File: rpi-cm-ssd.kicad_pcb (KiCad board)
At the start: 4 copper layers, 107 x 55.9 mm, 153 parts, among them J1 ARJM11B1-502-AB-EW2, J2 Bus_M.2_Socket_M, J3 USB_C_Receptacle, J4 PD controller EEPROM programm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, J5 690-008-221-904, J6 CONUFL001-SMD-T, Q1 DMG1012T, SW1 SW_DIP_x05, U1 SN74LVC1G11, U10 TPS65283-1RGER, U11 USB2512, U12 24LC32, U13 TCN75AVUA, U14 TCN75AVUA, U15 SN74LVC1G07, U16 MGM210PB32JIA2, U2 TPD4EUSB30, U3 TPD4EUSB30, U4 74LVC1G07, U5 SN74LVC1G3157, U6 CAT24C256, U7 TVS2200DRV, U8 TPS25750DRJKT, U9 PAC1951-1, Y1 24MHz

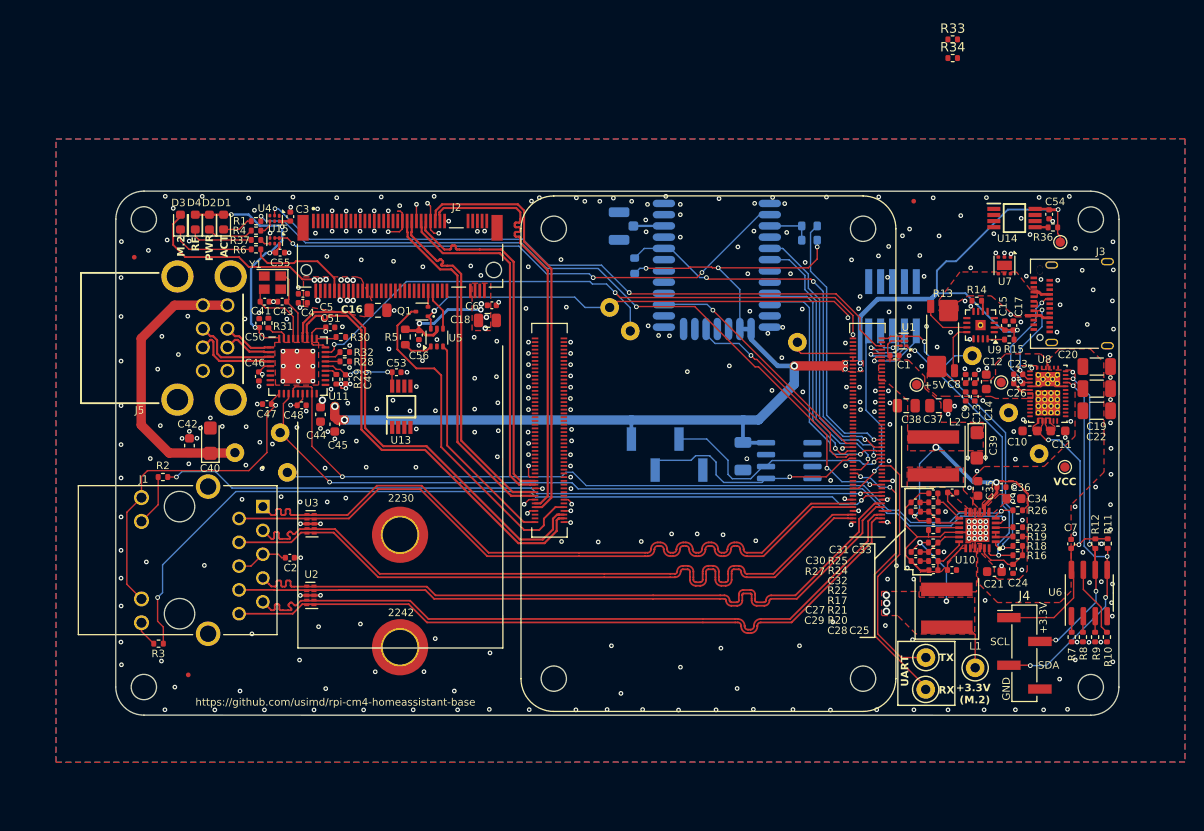
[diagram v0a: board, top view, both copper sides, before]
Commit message: Rev 2
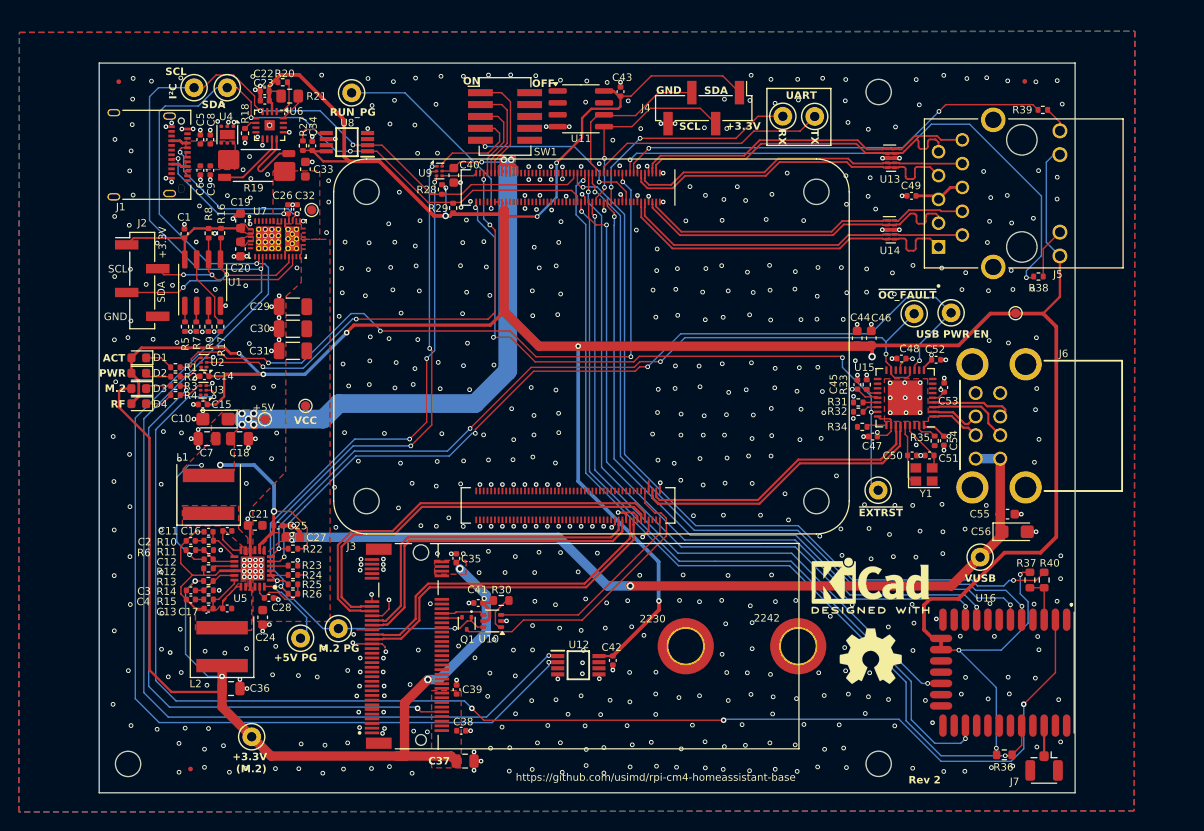
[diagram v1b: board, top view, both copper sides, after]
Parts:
- removed the C12 at (149.8, 50.5)
- removed the C13 at (149.8, 52.4)
- removed the H4 at (61.1, 33.5)
- added C5: 10nF, Capacitor_SMD:C_0402_1005Metric, F.Cu at (67.1, 25.0)
- added C6: 10nF, Capacitor_SMD:C_0402_1005Metric, F.Cu at (67.1, 28.3)
- added R20: 100k, Resistor_SMD:R_0402_1005Metric, F.Cu at (75.9, 18.9)
- added REF**: KiCad-Logo2_5mm_SilkScreen, Symbol:KiCad-Logo2_5mm_SilkScreen, F.Cu at (138.6, 72.6)
- added REF**: OSHW-Symbol_6.7x6mm_SilkScreen, Symbol:OSHW-Symbol_6.7x6mm_SilkScreen, F.Cu at (138.7, 80.1)
- added REF**: WEEE-Logo_4.2x6mm_SilkScreen, Symbol:WEEE-Logo_4.2x6mm_SilkScreen, B.Cu at (132.8, 90.2)
- added REF**: RoHS-Logo_6mm_SilkScreen, Symbol:RoHS-Logo_6mm_SilkScreen, B.Cu at (110.7, 90.4)
- added REF**: ESD-Logo_6.6x6mm_SilkScreen, Symbol:ESD-Logo_6.6x6mm_SilkScreen, B.Cu at (126.0, 90.4)
- added REF**: Symbol_GNU-Logo_SilkscreenTop, Symbol:Symbol_GNU-Logo_SilkscreenTop, B.Cu at (81.5, 86.0)
- C40: renamed from C1; footprint Capacitor_SMD:C_0402_1005Metric -> Capacitor_SMD:C_0603_1608Metric
- C43: renamed from C52; footprint Capacitor_SMD:C_1206_3216Metric -> Capacitor_SMD:C_0402_1005Metric; moved to F.Cu
- J4: renamed from J7; moved to F.Cu
- J7: renamed from J6; moved to F.Cu
- R21: renamed from R15; footprint Resistor_SMD:R_0402_1005Metric -> Resistor_SMD:R_0805_2012Metric
- R36: renamed from R40; moved to F.Cu
- R37: renamed from R39; moved to F.Cu
- R40: renamed from R38; moved to F.Cu
- SW1, U16: moved to F.Cu
- TP1: renamed from TP11; moved to F.Cu
- TP12: renamed from TP1; moved to F.Cu
- TP13: renamed from TP15; moved to F.Cu
- TP14: renamed from TP16; moved to F.Cu
- TP15: renamed from TP9; moved to F.Cu
- TP2: renamed from TP20; moved to F.Cu
- TP3: renamed from TP18; moved to F.Cu
- TP6: renamed from TP10; moved to F.Cu
- TP9: renamed from TP3; moved to F.Cu
- U11: renamed from U12; moved to F.Cu
- moved H2 118.0 mm to (59.4, 91.6)
- moved R39 110.2 mm to (157.0, 21.8), turned to 0 degrees
- moved J2 102.2 mm to (60.9, 40.0)
- moved J1 101.6 mm to (60.8, 26.6), turned to -90 degrees
- moved C1 100.2 mm to (65.4, 35.0)
- moved R16 100.2 mm to (69.3, 35.0)
- moved R5 100.2 mm to (65.5, 44.9)
- moved R8 100.2 mm to (68.0, 35.0)
- moved R9 100.2 mm to (68.0, 44.9)
- moved R17 100.2 mm to (69.3, 44.9)
- moved R7 100.2 mm to (66.7, 44.9)
- moved U1 100.2 mm to (67.4, 40.2)
- moved FID3 98.1 mm to (66.1, 92.1)
- moved J5 98.0 mm to (154.8, 30.7), turned to 90 degrees
- moved FID1 96.8 mm to (155.1, 18.8)
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- renumbered C7 to C1, C39 to C10, C31 to C11, C32 to C12, C28 to C13, C3 to C14, C55 to C15, C33 to C16, C25 to C17, C37 to C18, C10 to C19, C30 to C2, C11 to C20, C35 to C21, C17 to C22, C15 to C23, C21 to C24, C36 to C25, C34 to C27, C24 to C28, C22 to C29, C27 to C3, C19 to C30, C20 to C31, C23 to C32, C14 to C33, C54 to C34, C6 to C35, C18 to C36, C16 to C37, C5 to C38, C4 to C39, C29 to C4, C56 to C41, C53 to C42, C45 to C44, C49 to C45, C44 to C46, C51 to C47, C2 to C49, C43 to C50, C41 to C51, C47 to C52, C46 to C53, C50 to C54, C42 to C55, C40 to C56, C38 to C7, FID3 to FID2, FID2 to FID3, H3 to H2, H6 to H3, H5 to H4, H2 to H5, H1 to H6, J3 to J1, J4 to J2, J2 to J3, J1 to J5, J5 to J6, L2 to L1, L1 to L2, R25 to R10, R24 to R11, R22 to R12, R17 to R13, R21 to R14, R20 to R15, R11 to R16, R10 to R17, R14 to R18, R13 to R19, R4 to R2, R26 to R22, R19 to R24, R18 to R25, R16 to R26, R36 to R27, R34 to R28, R33 to R29, R6 to R3, R5 to R30, R28 to R31, R29 to R33, R30 to R34, R31 to R35, R2 to R38, R3 to R39, R37 to R4, R7 to R5, R27 to R6, R8 to R7, R12 to R8, TP4 to TP10, TP5 to TP11, TP2 to TP16, TP14 to TP4, TP13 to TP5, TP8 to TP7, TP12 to TP8, U6 to U1, U5 to U10, U13 to U12, U2 to U13, U3 to U14, U11 to U15, U4 to U2, U15 to U3, U7 to U4, U10 to U5, U9 to U6, U8 to U7, U14 to U8, U1 to U9
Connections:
- C8 pad 1: VBUS -> /Power/VIN
- C9 pad 1: VBUS -> /Power/VIN
- J5 pad 10: /CM4 GPIO/TRD3_P -> /CM4 GPIO/TRD3_N
- J5 pad 9: /CM4 GPIO/TRD3_N -> /CM4 GPIO/TRD3_P
- TP2 pad 1: /Sensors/I2C.SCL -> /CM4 GPIO/I2C.SCL
- TP3 pad 1: /Sensors/I2C.SDA -> /CM4 GPIO/I2C.SDA
- U12 pad 1: /Sensors/I2C.SDA -> /CM4 GPIO/I2C.SDA
- U12 pad 2: /Sensors/I2C.SCL -> /CM4 GPIO/I2C.SCL
- U13 pad 1: /CM4 GPIO/TRD3_P -> /CM4 GPIO/TRD3_N
- U13 pad 10: /CM4 GPIO/TRD3_P -> /CM4 GPIO/TRD3_N
- U13 pad 2: /CM4 GPIO/TRD3_N -> /CM4 GPIO/TRD3_P
- U13 pad 9: /CM4 GPIO/TRD3_N -> /CM4 GPIO/TRD3_P
- U6 pad 4: /Power/I2C.SCL -> /CM4 GPIO/I2C.SCL
- U6 pad 5: /Power/I2C.SDA -> /CM4 GPIO/I2C.SDA
- U7 pad 8: /Power/I2C.SDA -> /CM4 GPIO/I2C.SDA
- U7 pad 9: /Power/I2C.SCL -> /CM4 GPIO/I2C.SCL
- U8 pad 1: /Sensors/I2C.SDA -> /CM4 GPIO/I2C.SDA
- U8 pad 2: /Sensors/I2C.SCL -> /CM4 GPIO/I2C.SCL
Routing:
- net /CM4 GPIO/I2C.SCL: track 0.00 -> 182.5 mm, vias 0 -> 4
- net /CM4 GPIO/I2C.SDA: track 0.00 -> 177.7 mm, vias 0 -> 4
- net +3.3V: track 241.4 -> 381.5 mm, vias 23 -> 19
- net /Wireless/~{LED_WIRELESS}: track 57.4 -> 147.8 mm, vias 3 -> 4
- net +5V: track 31.9 -> 104.6 mm, vias 3 -> 12
- net /CM4 GPIO/Wireless.CTS: track 26.3 -> 85.3 mm, vias 1 -> 2
- net /CM4 GPIO/Wireless.~{BOOT}: track 28.2 -> 84.3 mm, vias 1 -> 2
- net Net-(J3-DAS/~{DSS}/~{LED1}): track 11.1 -> 66.6 mm, vias 0 -> 2
- net /CM4 GPIO/Wireless.~{RESET}: track 43.4 -> 96.9 mm, vias 3 -> 2
- net /CM4 GPIO/Wireless.RXD: track 23.8 -> 76.5 mm, vias 1 -> 2
- net /CM4 GPIO/Wireless.SWCLK: track 30.0 -> 82.5 mm, vias 1 -> 2
- net GND: track 54.4 -> 106.8 mm, vias 408 -> 721
- net /CM4 GPIO/Wireless.RTS: track 22.9 -> 75.1 mm, vias 1 -> 2
- net /CM4 GPIO/Wireless.TXD: track 26.7 -> 78.5 mm, vias 1 -> 2
- net /CM4 GPIO/Wireless.SWDIO: track 30.1 -> 78.1 mm, vias 1 -> 2
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- added copper zone on B.Cu, net +5V
- removed copper zone on F.Cu, net +3.3V
- removed copper zone on In2.Cu, net +3V3
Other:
- board size 107 x 55.9 mm -> 104.1 x 77.9 mm
- board text added: "I²C"
- board text added: "Rev 2"
- board text removed: "I2C_SCL"
- board text removed: "I2C_SDA"
